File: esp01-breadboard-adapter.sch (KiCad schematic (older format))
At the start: 4 parts, among them P1 CONN_02X04, P2 CONN_01X04, P3 CONN_01X04

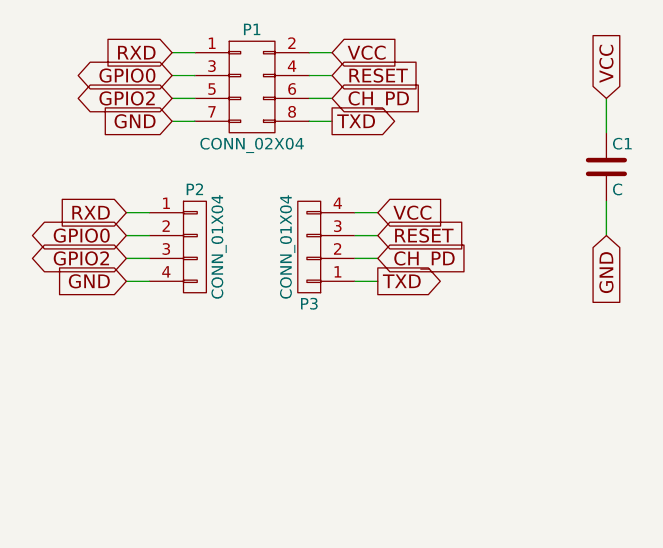
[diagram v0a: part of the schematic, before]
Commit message: begin 2nd layer pcb
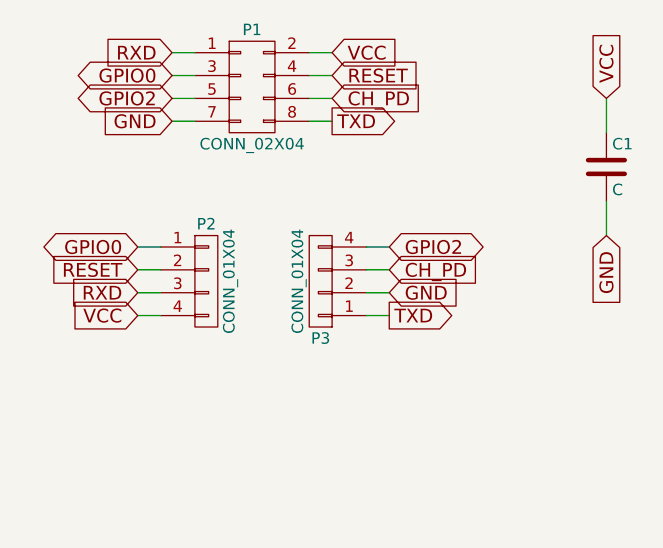
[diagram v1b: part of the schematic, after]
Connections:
- net CH_PD: now also P3.3 (P3); no longer P3.2 (P2)
- net GND: now also P3.2 (P2); no longer P2.4 (P4)
- net GPIO0: now also P2.1 (P1); no longer P2.2 (P2)
- net GPIO2: now also P3.4 (P4); no longer P2.3 (P3)
- net RESET: now also P2.2 (P2); no longer P3.3 (P3)
- net RXD: now also P2.3 (P3); no longer P2.1 (P1)
- net VCC: now also P2.4 (P4); no longer P3.4 (P4)
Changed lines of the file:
@@
-GND
-$Comp
-L CONN_01X04 P3
-U 1 1 585E6908
-P 5900 4000
-F 0 "P3" H 5900 4250 50  0000 C CNN
-F 1 "CONN_01X04" V 6000 4000 50  0000 C CNN
-F 2 "Pin_Headers:Pin_Header_Straight_1x04" H 5900 4000 50  0001 C CNN
-F 3 "" H 5900 4000 50  0000 C CNN
-	1    5900 4000
-	-1   0    0    1
-$EndComp
-$Comp
-L CONN_01X04 P2
-U 1 1 585E69F1
-P 5400 4000
-F 0 "P2" H 5400 4250 50  0000 C CNN
-F 1 "CONN_01X04" V 5500 4000 50  0000 C CNN
-F 2 "Pin_Headers:Pin_Header_Straight_1x04" H 5400 4000 50  0001 C CNN
-F 3 "" H 5400 4000 50  0000 C CNN
-	1    5400 4000
-	1    0    0    -1
-$EndComp
-Wire Wire Line
-	6100 3850 6200 3850
-Wire Wire Line
-	6100 3950 6200 3950
-Wire Wire Line
-	6100 4050 6200 4050
-Wire Wire Line
-	6100 4150 6200 4150
-Text GLabel 6200 3850 2    60   Input ~ 0
-VCC
-Text GLabel 6200 3950 2    60   Input ~ 0
-RESET
-Text GLabel 6200 4050 2    60   Input ~ 0
-CH_PD
-Text GLabel 6200 4150 2    60   Output ~ 0
-TXD
-Wire Wire Line
-	5200 4150 5100 4150
-Wire Wire Line
-	5200 4050 5100 4050
-Wire Wire Line
-	5200 3950 5100 3950
-Wire Wire Line
-	5200 3850 5100 3850
-Text GLabel 5100 3850 0    60   Input ~ 0
-RXD
-Text GLabel 5100 3950 0    60   BiDi ~ 0
-GPIO0
-Text GLabel 5100 4050 0    60   BiDi ~ 0
-GPIO2
-Text GLabel 5100 4150 0    60   Input ~ 0
 GND
 $Comp
@@
 Text Notes 7450 7250 0    60   ~ 0
 Francesco Urbani\n
+$Comp
+L CONN_01X04 P3
+U 1 1 585F9D0E
+P 5950 4150
+F 0 "P3" H 5950 4400 50  0000 C CNN
+F 1 "CONN_01X04" V 6050 4150 50  0000 C CNN
+F 2 "Pin_Headers:Pin_Header_Straight_1x04" H 5950 4150 50  0001 C CNN
+F 3 "" H 5950 4150 50  0000 C CNN
+	1    5950 4150
+	-1   0    0    1
+$EndComp
+$Comp
+L CONN_01X04 P2
+U 1 1 585F9D14
+P 5450 4150
+F 0 "P2" H 5450 4400 50  0000 C CNN
+F 1 "CONN_01X04" V 5550 4150 50  0000 C CNN
+F 2 "Pin_Headers:Pin_Header_Straight_1x04" H 5450 4150 50  0001 C CNN
+F 3 "" H 5450 4150 50  0000 C CNN
+	1    5450 4150
+	1    0    0    -1
+$EndComp
+Wire Wire Line
+	6150 4000 6250 4000
+Wire Wire Line
+	6150 4100 6250 4100
+Wire Wire Line
+	6150 4200 6250 4200
+Wire Wire Line
+	6150 4300 6250 4300
+Text GLabel 6250 4000 2    60   BiDi ~ 0
+GPIO2
+Text GLabel 6250 4100 2    60   Input ~ 0
+CH_PD
+Text GLabel 6250 4200 2    60   Input ~ 0
+GND
+Text GLabel 6250 4300 2    60   Output ~ 0
+TXD
+Wire Wire Line
+	5250 4300 5150 4300
+Wire Wire Line
+	5250 4200 5150 4200
+Wire Wire Line
+	5250 4100 5150 4100
+Wire Wire Line
+	5250 4000 5150 4000
+Text GLabel 5150 4000 0    60   BiDi ~ 0
+GPIO0
+Text GLabel 5150 4100 0    60   Input ~ 0
+RESET
+Text GLabel 5150 4200 0    60   Input ~ 0
+RXD
+Text GLabel 5150 4300 0    60   Input ~ 0
+VCC
 $EndSCHEMATC
